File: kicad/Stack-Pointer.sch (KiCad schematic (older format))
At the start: 8 parts, among them U100 74LS86, U101 74LS191, U102 74LS191, U95 74LS86, U96 74LS191, U97 74LS245, U98 74LS191, U99 74LS245

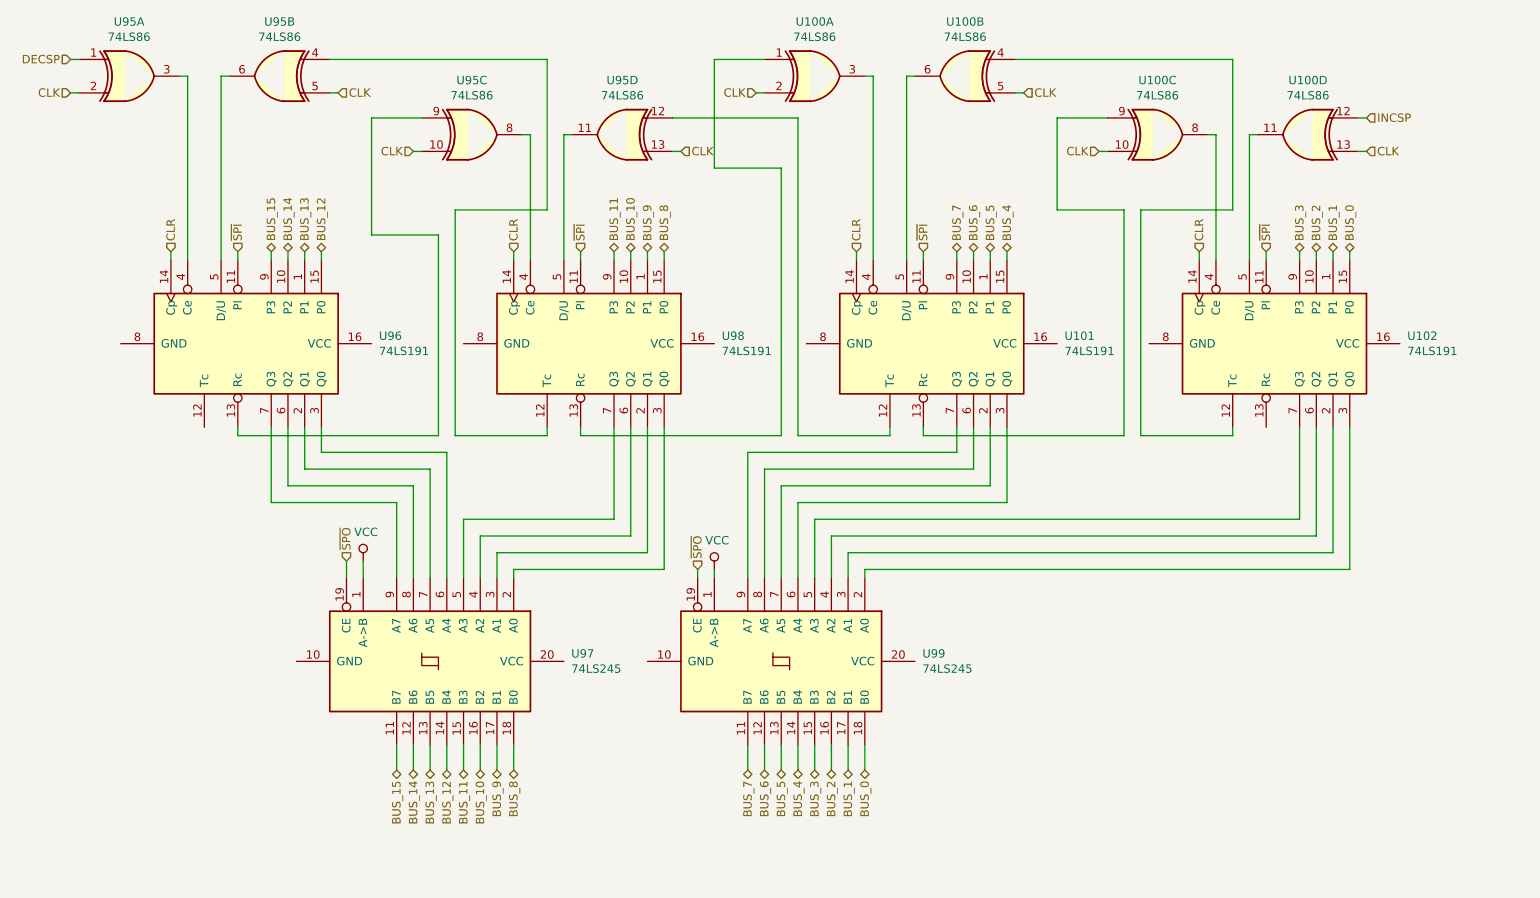
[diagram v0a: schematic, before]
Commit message: Up to v1.0 and plot
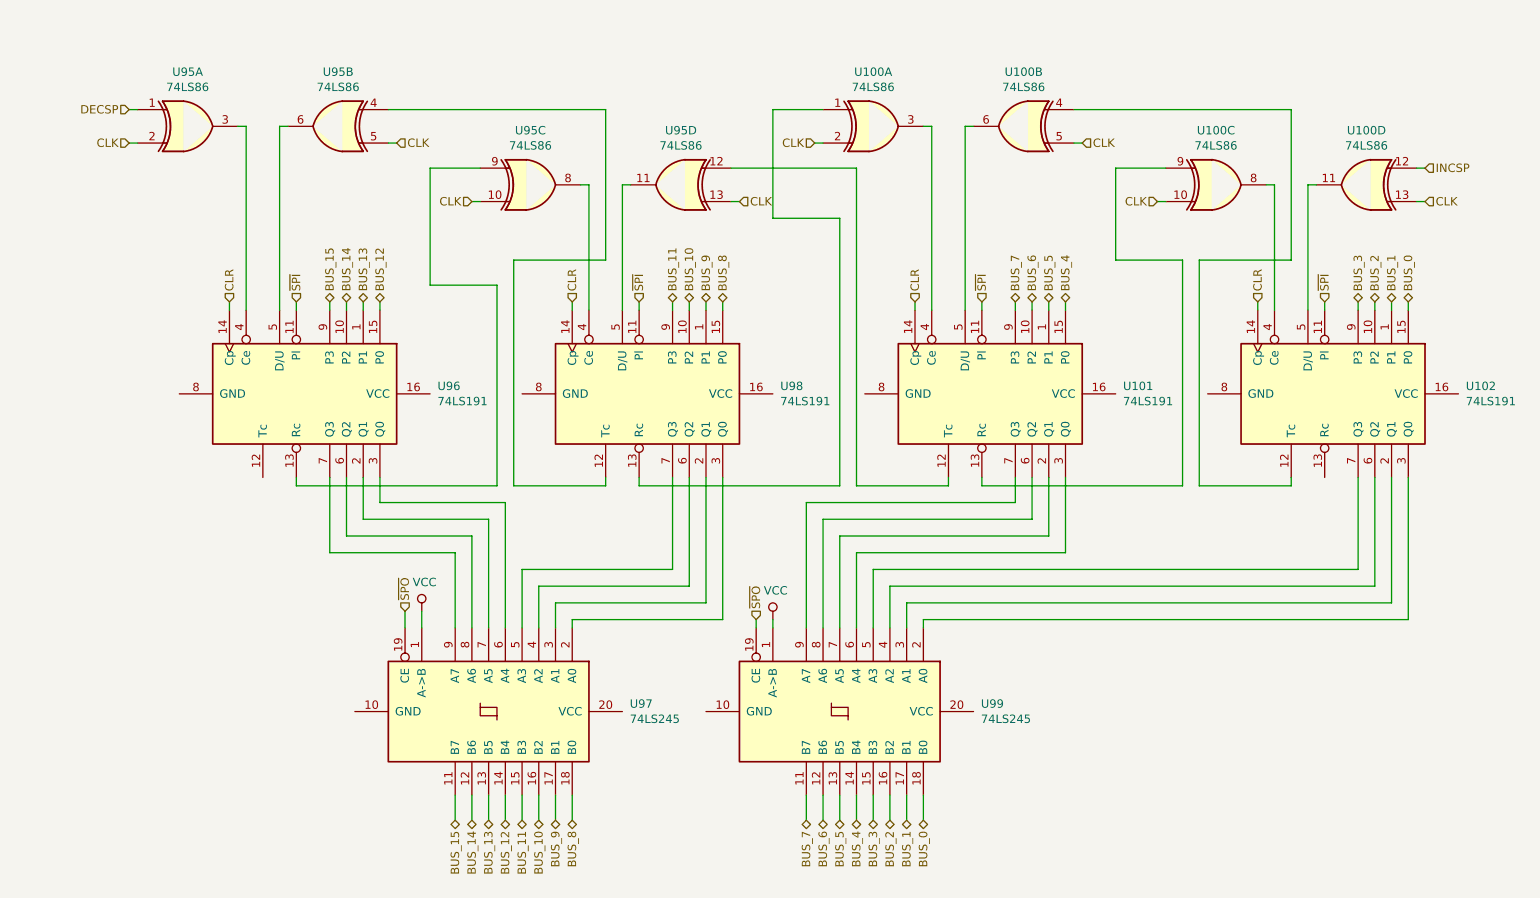
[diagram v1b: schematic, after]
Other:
- moved on the sheet: U100A, U100B, U100C, U100D, U101, U102, U95A, U95B, U95C, U95D, U96, U97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
